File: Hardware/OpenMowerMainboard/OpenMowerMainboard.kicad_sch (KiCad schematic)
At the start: 9 parts, among them U1 LM2596S_MODULE

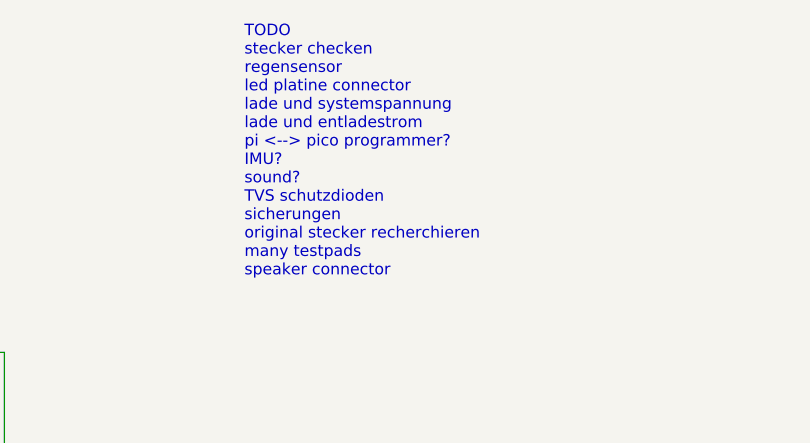
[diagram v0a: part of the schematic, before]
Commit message: wip schematic
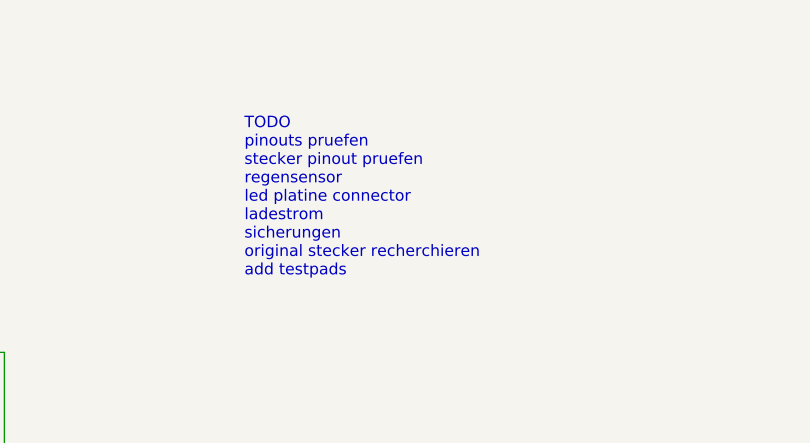
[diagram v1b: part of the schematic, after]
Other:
- note added: "TODO pinouts pruefen stecker pinout pruefen regensensor led platine connector ladestrom sicherungen original stecker recherchieren add testpads"
- note removed: "TODO stecker checken regensensor led platine connector lade und systemspannung lade und entladestrom pi <--> pico programmer? IMU? sound? TVS schutzdioden sicherungen original stecker recherchieren many testpads speaker connector"
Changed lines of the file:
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@@
     (effects (font (size 1.27 1.27)) (justify left bottom))
   )
-  (text "TODO\nstecker checken\nregensensor\nled platine connector\nlade und systemspannung\nlade und entladestrom\npi <--> pico programmer?\nIMU?\nsound?\nTVS schutzdioden\nsicherungen\noriginal stecker recherchieren\nmany testpads\nspeaker connector"
+  (text "TODO\npinouts pruefen\nstecker pinout pruefen\nregensensor\nled platine connector\nladestrom\nsicherungen\noriginal stecker recherchieren\nadd testpads"
     (at 288.29 66.675 0)
     (effects (font (size 1.27 1.27)) (justify left bottom))
@@
       (reference "D3") (unit 1) (value "D_Schottky") (footprint "")
     )
+    (path "/a66eb396-0410-43f5-a37d-ef2abb980a3a/4ebdc7ab-25b0-4467-9229-087b84fdf66f"
+      (reference "D4") (unit 1) (value "D_TVS") (footprint "Diode_SMD:D_SMB")
+    )
+    (path "/a66eb396-0410-43f5-a37d-ef2abb980a3a/55b8a13b-6894-4208-a000-86cbaab261aa"
+      (reference "D5") (unit 1) (value "D_TVS") (footprint "Diode_SMD:D_SMB")
+    )
+    (path "/a66eb396-0410-43f5-a37d-ef2abb980a3a/37a9969b-e03a-4c0a-94f9-c1bfb2bcb429"
+      (reference "D6") (unit 1) (value "D_TVS") (footprint "Diode_SMD:D_SMB")
+    )
+    (path "/a66eb396-0410-43f5-a37d-ef2abb980a3a/56203402-79b1-40a1-97ad-4c42312e0916"
+      (reference "D7") (unit 1) (value "D_TVS") (footprint "Diode_SMD:D_SMB")
+    )
+    (path "/a66eb396-0410-43f5-a37d-ef2abb980a3a/dcbf07c1-fd83-46b4-9cb8-68d7fd77aad4"
+      (reference "D8") (unit 1) (value "D_TVS") (footprint "Diode_SMD:D_SMB")
+    )
+    (path "/a66eb396-0410-43f5-a37d-ef2abb980a3a/8d636e49-195d-4662-8b69-230d986a3b72"
+      (reference "D9") (unit 1) (value "D_TVS") (footprint "Diode_SMD:D_SMB")
+    )
+    (path "/a66eb396-0410-43f5-a37d-ef2abb980a3a/2bebeb4d-3b78-44b1-9d84-649cd389bb68"
+      (reference "D10") (unit 1) (value "D_TVS") (footprint "Diode_SMD:D_SMB")
+    )
+    (path "/a66eb396-0410-43f5-a37d-ef2abb980a3a/20b8b1d3-3d67-4311-99ca-ce5363c0cad0"
+      (reference "D11") (unit 1) (value "D_TVS") (footprint "Diode_SMD:D_SMB")
+    )
+    (path "/a66eb396-0410-43f5-a37d-ef2abb980a3a/a6025457-ad02-406e-ac1d-03834a754964"
+      (reference "D12") (unit 1) (value "D_TVS") (footprint "Diode_SMD:D_SMB")
+    )
+    (path "/00000000-0000-0000-0000-000061040c60/520089b0-4442-4713-ae1b-87d63d51b467"
+      (reference "F1") (unit 1) (value "Fuse") (footprint "MyModules:Fuseholder5x20_horiz_open_inline_Type-I")
+    )
+    (path "/00000000-0000-0000-0000-000061040c60/b9168f77-b5a5-4161-8a9b-951a2e8475d3"
+      (reference "F2") (unit 1) (value "Fuse") (footprint "MyModules:Fuseholder5x20_horiz_open_inline_Type-I")
+    )
+    (path "/00000000-0000-0000-0000-000061040c60/89a9550d-36a5-40f8-a465-c83bb62d834f"
+      (reference "F3") (unit 1) (value "Fuse") (footprint "MyModules:Fuseholder5x20_horiz_open_inline_Type-I")
+    )
+    (path "/00000000-0000-0000-0000-000061040c60/58391851-bdb9-4e0a-bc80-50f6a07fc993"
+      (reference "F4") (unit 1) (value "Fuse") (footprint "MyModules:Fuseholder5x20_horiz_open_inline_Type-I")
+    )
     (path "/00000000-0000-0000-0000-000060ffea54"
       (reference "H1") (unit 1) (value "MountingHole_Pad") (footprint "MountingHole:MountingHole_5mm_Pad")
@@
       (reference "J10") (unit 1) (value "Conn_01x05") (footprint "Connector_JST:JST_PH_B5B-PH-K_1x05_P2.00mm_Vertical")
     )
-    (path "/df7e4e30-b8d5-4f4b-a24f-39298e982d26/00000000-0000-0000-0000-00006130130c"
-      (reference "J11") (unit 1) (value "Conn_01x10_Female") (footprint "Connector_PinHeader_2.54mm:PinHeader_1x10_P2.54mm_Vertical")
-    )
     (path "/00000000-0000-0000-0000-000061040c60/b1812e93-6d07-48bc-8440-4307c7b13cf3"
       (reference "J11") (unit 1) (value "Conn_01x03_Male") (footprint "Connector_JST:JST_XH_B3B-XH-A_1x03_P2.50mm_Vertical")
@@
       (reference "J19") (unit 1) (value "Conn_01x04") (footprint "Connector_JST:JST_XH_B4B-XH-A_1x04_P2.50mm_Vertical")
     )
+    (path "/df7e4e30-b8d5-4f4b-a24f-39298e982d26/00000000-0000-0000-0000-00006130130c"
+      (reference "J20") (unit 1) (value "Conn_01x10_Female") (footprint "Connector_PinHeader_2.54mm:PinHeader_1x10_P2.54mm_Vertical")
+    )
     (path "/00000000-0000-0000-0000-00006109dce5/06715042-9807-4840-bc8e-1cf593cdbcdf"
       (reference "JP1") (unit 1) (value "SolderJumper_3_Bridged12") (footprint "")
@@
       (reference "R50") (unit 1) (value "10k") (footprint "Resistor_THT:R_Axial_DIN0309_L9.0mm_D3.2mm_P12.70mm_Horizontal")
     )
+    (path "/00000000-0000-0000-0000-000061040c60/f11b3e3a-7b08-49d8-b4b1-92030ffe70c2"
+      (reference "R51") (unit 1) (value "R") (footprint "Resistor_SMD:R_Shunt_Vishay_WSK2512_6332Metric_T2.66mm")
+    )
     (path "/989a400d-9ce2-403e-a19e-ad0a758fe27c/b948dd43-413f-4002-adce-e082c45a5179"
       (reference "R53") (unit 1) (value "1k5") (footprint "Resistor_THT:R_Axial_DIN0309_L9.0mm_D3.2mm_P12.70mm_Horizontal")
@@
       (reference "R57") (unit 1) (value "27k") (footprint "Resistor_THT:R_Axial_DIN0309_L9.0mm_D3.2mm_P12.70mm_Horizontal")
     )
-    (path "/00000000-0000-0000-0000-000061040c60/f11b3e3a-7b08-49d8-b4b1-92030ffe70c2"
-      (reference "R?") (unit 1) (value "R") (footprint "Resistor_SMD:R_Shunt_Vishay_WSK2512_6332Metric_T2.66mm")
-    )
     (path "/989a400d-9ce2-403e-a19e-ad0a758fe27c/88528529-64b3-4d79-b2db-e04c4b468443"
